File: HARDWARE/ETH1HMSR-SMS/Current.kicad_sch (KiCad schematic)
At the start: 40 parts, among them J501 1710072, U501 HMSR-SMS, U502 DG412LEDQ, U503 DG419LEDY, U504 DG412LEDQ, U505 OPA341UA, U506 OPA341UA, U507 OPA341UA

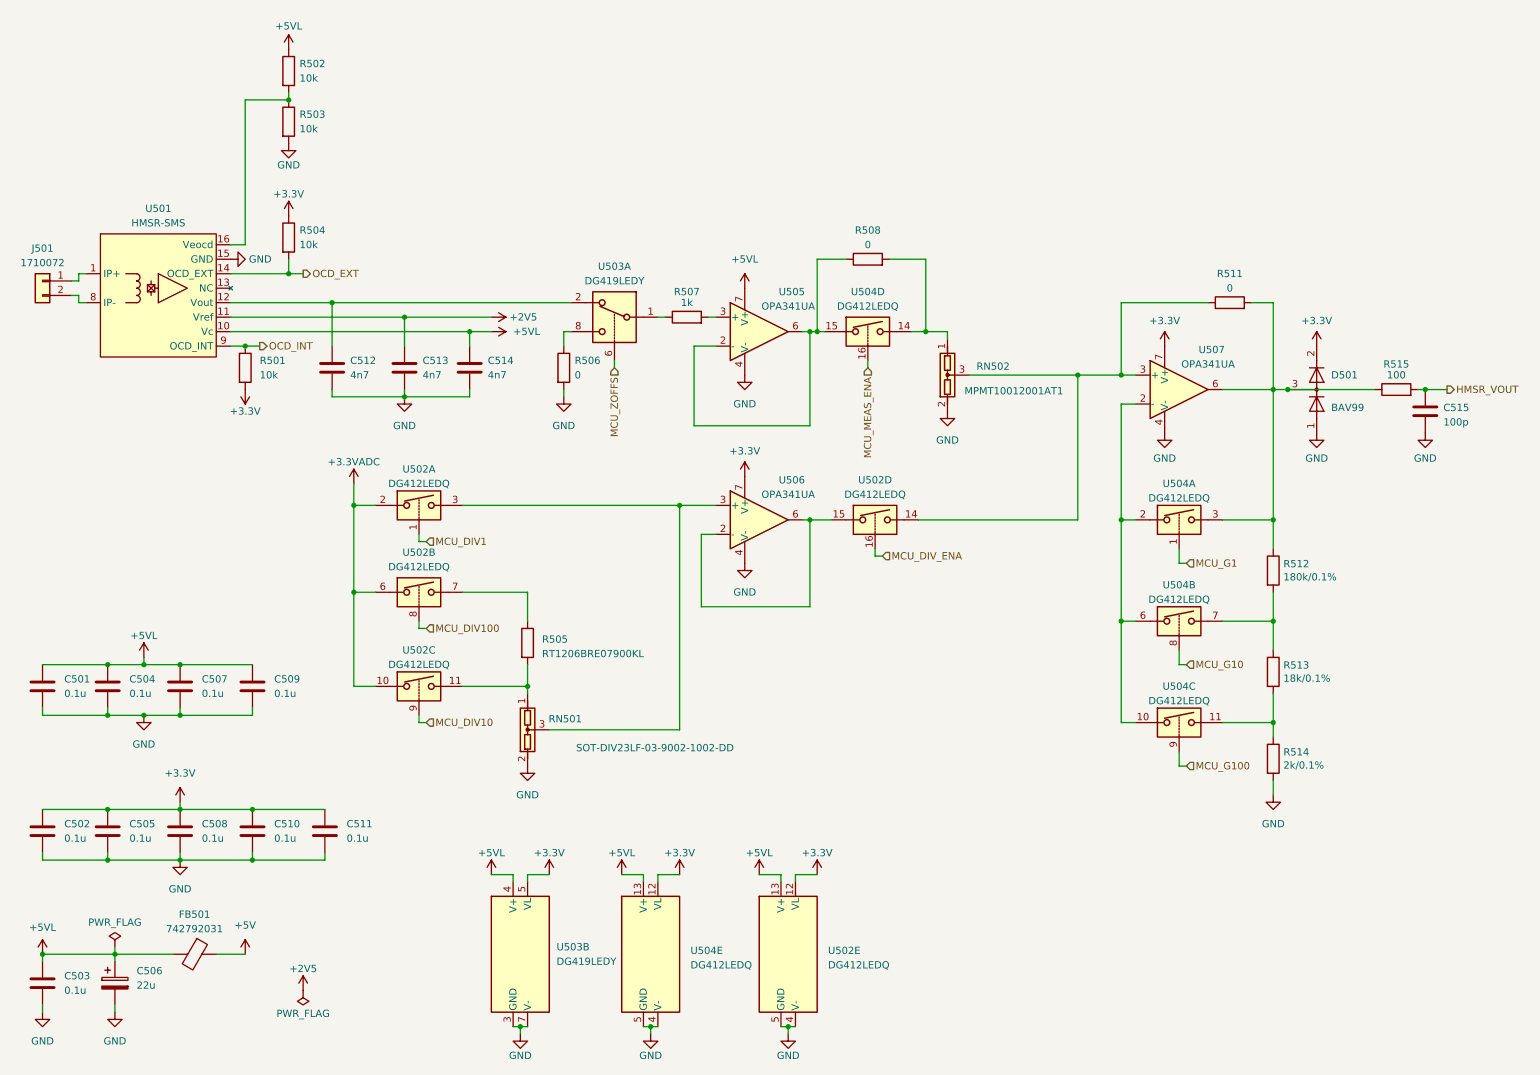
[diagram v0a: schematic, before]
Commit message: Development
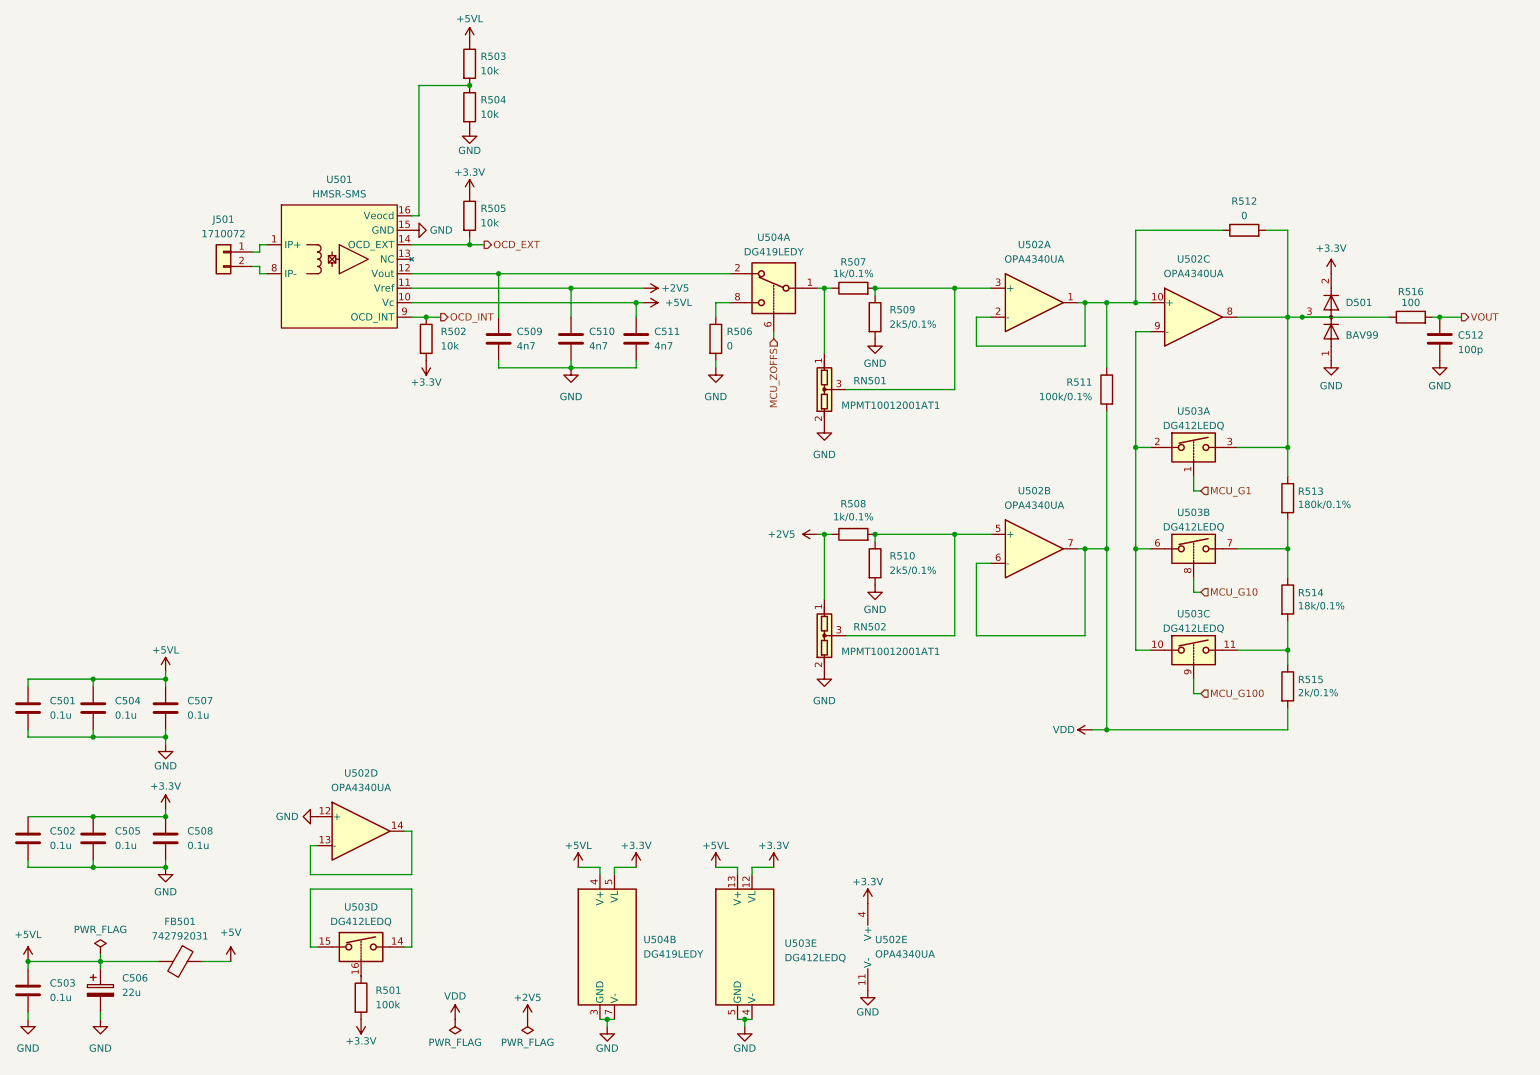
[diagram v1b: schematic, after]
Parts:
- removed C509, C510, C511: 0.1u, Capacitor_SMD:C_0603_1608Metric_Pad1.08x0.95mm_HandSolder, symbol Device:C
- removed R505: RT1206BRE07900KL, Resistor_SMD:R_1206_3216Metric_Pad1.30x1.75mm_HandSolder, symbol Device:R
- removed U502: DG412LEDQ, Package_SO:TSSOP-16_4.4x5mm_P0.65mm, symbol Analog_Switch:DG412xUE
- removed U505, U506, U507: OPA341UA, Package_SO:SOIC-8_3.9x4.9mm_P1.27mm, symbol Amplifier_Operational:OPA340UA
- added R501: 100k, Resistor_SMD:R_0603_1608Metric_Pad0.98x0.95mm_HandSolder, symbol Device:R
- added R509, R510: 2k5/0.1%, Resistor_SMD:R_0603_1608Metric_Pad0.98x0.95mm_HandSolder, symbol Device:R
- added R511: 100k/0.1%, Resistor_SMD:R_0603_1608Metric_Pad0.98x0.95mm_HandSolder, symbol Device:R
- added U502: OPA4340UA, Package_SO:SSOP-16_3.9x4.9mm_P0.635mm, symbol Amplifier_Operational:OPA4340UA
- R507: value 1k -> 1k/0.1%
- R508: value 0 -> 1k/0.1%
- RN501: value SOT-DIV23LF-03-9002-1002-DD -> MPMT10012001AT1
- renumbered C512 to C509, C513 to C510, C514 to C511, C515 to C512, R501 to R502, R502 to R503, R503 to R504, R504 to R505, R511 to R512, R512 to R513, R513 to R514, R514 to R515, R515 to R516, U504 to U503, U503 to U504
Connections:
- net +2V5: now also R508.1, RN502.1
- net +3.3V: now also R501.2, U502.4 (V+)
- net GND: now also R509.2, R510.2, U502.11 (V-), U502.12 (+); no longer R515.2
- net at U503.10, U503.2, U503.6: now also U502.9 (-)
- net at R512.1: now also R511.1, U502.1, U502.10 (+), U502.2 (-); no longer RN502.3
- net at D501.3 (K), R512.2, R513.1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: now also U502.8
- net at RN501.3: now also R507.2, R509.1, U502.3 (+)
- net at RN501.1: now also R507.1, U504.1
- net at U503.15: now also U503.14; no longer R508.1
- net HMSR_VOUT renamed VOUT
- net MCU_MEAS_ENA: no longer names the net of U503.16
- net MCU_MEAS_ENA: now also R501.1
- new net: U502.13 (-), U502.14
- new net: R508.2, R510.1, RN502.3, U502.5 (+)
- new net VDD: R511.2, R515.2, U502.6 (-), U502.7
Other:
- moved on the sheet: C501, C502, C503, C504, C505, C506, C507, C508, C509, C510, C511, C512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
